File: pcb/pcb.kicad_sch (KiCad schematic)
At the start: 0 parts

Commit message: initial pcb
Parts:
- added D1, D10, D11, D12, D13, D14, D15, D16, D17, D18, D19, D2, D20, D21, D22, D23, D24, D25, D26, D27, D28, D29, D3, D30, D31, D32, D33, D34, D35, D36, D37, D38, D39, D4, D40, D41, D42, D43, D44, D45, D46, D47, D48, D5, D6, D7, D8, D9: 1N4148, Diode_SMD:D_SOD-123, symbol Diode:1N4148
- added SW1, SW10, SW11, SW12, SW13, SW14, SW15, SW16, SW17, SW18, SW19, SW2, SW20, SW21, SW22, SW23, SW24, SW25, SW26, SW27, SW28, SW29, SW3, SW30, SW31, SW32, SW33, SW34, SW35, SW36, SW37, SW38, SW39, SW4, SW40, SW41, SW42, SW43, SW44, SW45, SW46, SW47, SW48, SW5, SW6, SW7, SW8, SW9: SW_SPST, keyswitches:SW_PG1350, symbol Switch:SW_SPST
- added SW49: SW_SPDT, symbol Switch:SW_SPDT
- added U1: SuperMini nRF52840, PCM_marbastlib-xp-promicroish:SuperMini_nRF52840_AH_USBdn, symbol PCM_marbastlib-promicroish:SuperMini_nRF52840
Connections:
- new net: D46.2 (A), SW46.1 (A)
- new net: D3.2 (A), SW3.1 (A)
- new net: D10.2 (A), SW10.1 (A)
- new net: D9.2 (A), SW9.1 (A)
- new net: D16.2 (A), SW16.1 (A)
- new net: D12.2 (A), SW12.1 (A)
- new net: D18.2 (A), SW18.1 (A)
- new net: D44.2 (A), SW44.1 (A)
- new net: D17.2 (A), SW17.1 (A)
- new net: D13.2 (A), SW13.1 (A)
- new net: D43.2 (A), SW43.1 (A)
- new net: D48.2 (A), SW48.1 (A)
- new net: D26.2 (A), SW26.1 (A)
- new net: D14.2 (A), SW14.1 (A)
- new net: D35.2 (A), SW35.1 (A)
- new net: D34.2 (A), SW34.1 (A)
- new net: D22.2 (A), SW22.1 (A)
- new net: D24.2 (A), SW24.1 (A)
- new net: D20.2 (A), SW20.1 (A)
- new net: D47.2 (A), SW47.1 (A)
- new net: D6.2 (A), SW6.1 (A)
- new net: D41.2 (A), SW41.1 (A)
- new net: D1.2 (A), SW1.1 (A)
- new net: D27.2 (A), SW27.1 (A)
- new net: D38.2 (A), SW38.1 (A)
- new net: D7.2 (A), SW7.1 (A)
- new net: D40.2 (A), SW40.1 (A)
- new net: D2.2 (A), SW2.1 (A)
- new net: D25.2 (A), SW25.1 (A)
- new net: D45.2 (A), SW45.1 (A)
- new net: D4.2 (A), SW4.1 (A)
- new net: D32.2 (A), SW32.1 (A)
- new net: D5.2 (A), SW5.1 (A)
- new net: D21.2 (A), SW21.1 (A)
- new net: D11.2 (A), SW11.1 (A)
- new net: D39.2 (A), SW39.1 (A)
- new net: D30.2 (A), SW30.1 (A)
- new net: D23.2 (A), SW23.1 (A)
- new net: D36.2 (A), SW36.1 (A)
- new net: D37.2 (A), SW37.1 (A)
- new net: D19.2 (A), SW19.1 (A)
- new net: D33.2 (A), SW33.1 (A)
- new net: D8.2 (A), SW8.1 (A)
- new net: D15.2 (A), SW15.1 (A)
- new net: D31.2 (A), SW31.1 (A)
- new net: D42.2 (A), SW42.1 (A)
- new net: D28.2 (A), SW28.1 (A)
- new net: D29.2 (A), SW29.1 (A)
- new net: U1.13 (BAT+), U1.29 (BAT+)
- new net col0: SW1.2 (B), SW13.2 (B), SW25.2 (B), SW37.2 (B)
- new net col1: SW14.2 (B), SW2.2 (B), SW26.2 (B), SW38.2 (B)
- new net col10: SW11.2 (B), SW23.2 (B), SW35.2 (B), SW47.2 (B)
- new net col11: SW12.2 (B), SW24.2 (B), SW36.2 (B), SW48.2 (B)
- new net col2: SW15.2 (B), SW27.2 (B), SW3.2 (B), SW39.2 (B)
- new net col3: SW16.2 (B), SW28.2 (B), SW4.2 (B), SW40.2 (B)
- new net col4: SW17.2 (B), SW29.2 (B), SW41.2 (B), SW5.2 (B)
- new net col5: SW18.2 (B), SW30.2 (B), SW42.2 (B), SW6.2 (B)
- new net col6: SW19.2 (B), SW31.2 (B), SW43.2 (B), SW7.2 (B)
- new net col7: SW20.2 (B), SW32.2 (B), SW44.2 (B), SW8.2 (B)
- new net col8: SW21.2 (B), SW33.2 (B), SW45.2 (B), SW9.2 (B)
- new net col9: SW10.2 (B), SW22.2 (B), SW34.2 (B), SW46.2 (B)
- new net row0: D1.1 (K), D10.1 (K), D11.1 (K), D12.1 (K), D2.1 (K), D3.1 (K), D4.1 (K), D5.1 (K), D6.1 (K), D7.1 (K), D8.1 (K), D9.1 (K)
- new net row1: D13.1 (K), D14.1 (K), D15.1 (K), D16.1 (K), D17.1 (K), D18.1 (K), D19.1 (K), D20.1 (K), D21.1 (K), D22.1 (K), D23.1 (K), D24.1 (K)
- new net row2: D25.1 (K), D26.1 (K), D27.1 (K), D28.1 (K), D29.1 (K), D30.1 (K), D31.1 (K), D32.1 (K), D33.1 (K), D34.1 (K), D35.1 (K), D36.1 (K)
- new net row3: D37.1 (K), D38.1 (K), D39.1 (K), D40.1 (K), D41.1 (K), D42.1 (K), D43.1 (K), D44.1 (K), D45.1 (K), D46.1 (K), D47.1 (K), D48.1 (K)

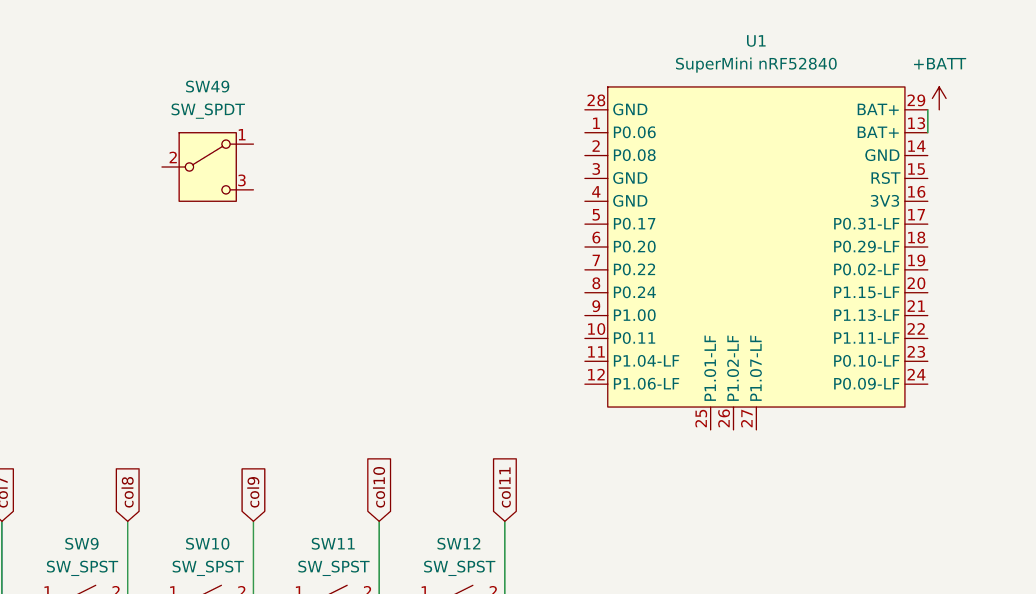
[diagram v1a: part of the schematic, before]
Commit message: pcb v1 done
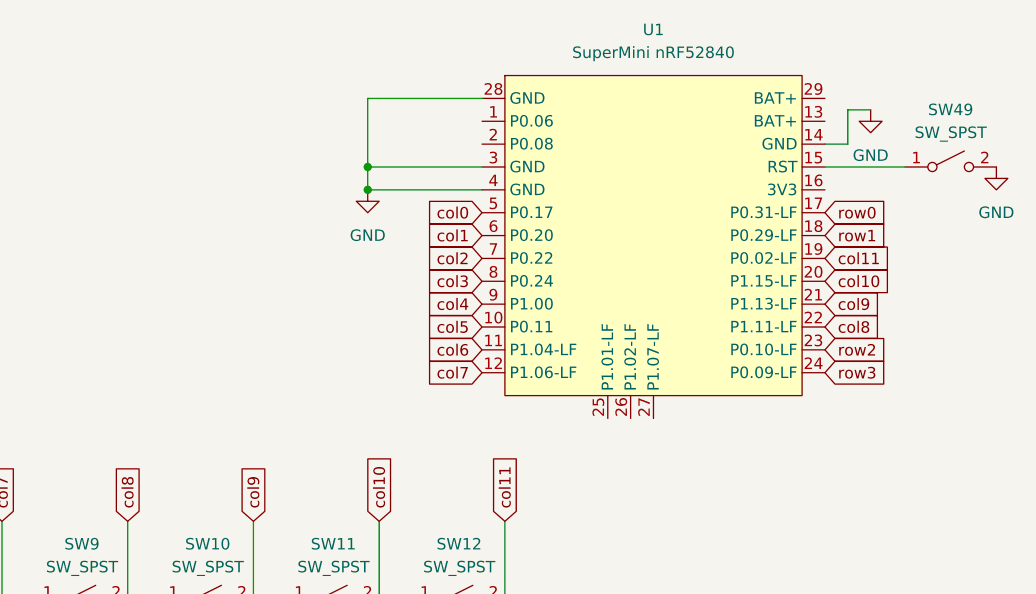
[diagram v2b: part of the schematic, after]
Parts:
- removed SW49: SW_SPDT, symbol Switch:SW_SPDT
- added SW49: SW_SPST, TS-1088-AR02016:SW_TS-1088-AR02016, symbol Switch:SW_SPST
- U1: footprint PCM_marbastlib-xp-promicroish:SuperMini_nRF52840_AH_USBdn -> PCM_marbastlib-xp-promicroish:SuperMini_nRF52840_H_USBdn
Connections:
- net col0: now also U1.5 (P0.17)
- net col1: now also U1.6 (P0.20)
- net col10: now also U1.20 (P1.15-LF)
- net col11: now also U1.19 (P0.02-LF)
- net col2: now also U1.7 (P0.22)
- net col3: now also U1.8 (P0.24)
- net col4: now also U1.9 (P1.00)
- net col5: now also U1.10 (P0.11)
- net col6: now also U1.11 (P1.04-LF)
- net col7: now also U1.12 (P1.06-LF)
- net col8: now also U1.22 (P1.11-LF)
- net col9: now also U1.21 (P1.13-LF)
- net row0: now also U1.17 (P0.31-LF)
- net row1: now also U1.18 (P0.29-LF)
- net row2: now also U1.23 (P0.10-LF)
- net row3: now also U1.24 (P0.09-LF)
- net at U1.13 (BAT+): no longer U1.29 (BAT+)
- net GND: now reaches U1.14 (GND)
- net GND: now also U1.28 (GND), U1.3 (GND), U1.4 (GND), SW49.2 (B)
- net at U1.15 (RST): now also SW49.1 (A)
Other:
- moved on the sheet: U1

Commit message: small schematic changes
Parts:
- SW49: LCSC (none) -> C720477
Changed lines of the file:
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@@
+			)
+		)
+		(property "LCSC" "C720477"
+			(at 270.51 33.02 0)
+			(effects
+				(font
+					(size 1.27 1.27)
+				)
+				(hide yes)
 			)
 		)
